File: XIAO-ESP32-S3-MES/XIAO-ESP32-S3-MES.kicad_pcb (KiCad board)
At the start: 2 copper layers, 36 x 39 mm, 11 parts, among them SW1 Conn_01x02_Socket, U2 XIAO-ESP32-S3-SMD

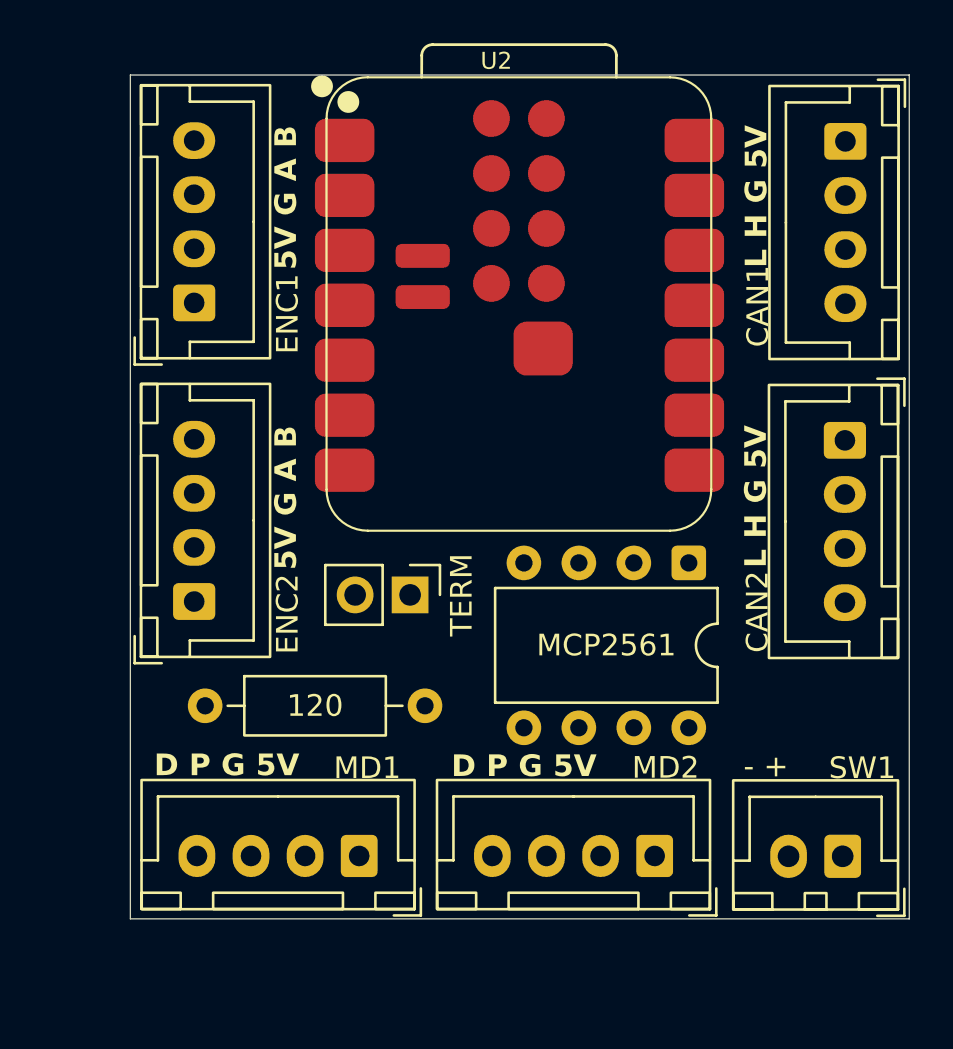
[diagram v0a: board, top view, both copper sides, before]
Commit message: MES配置完了
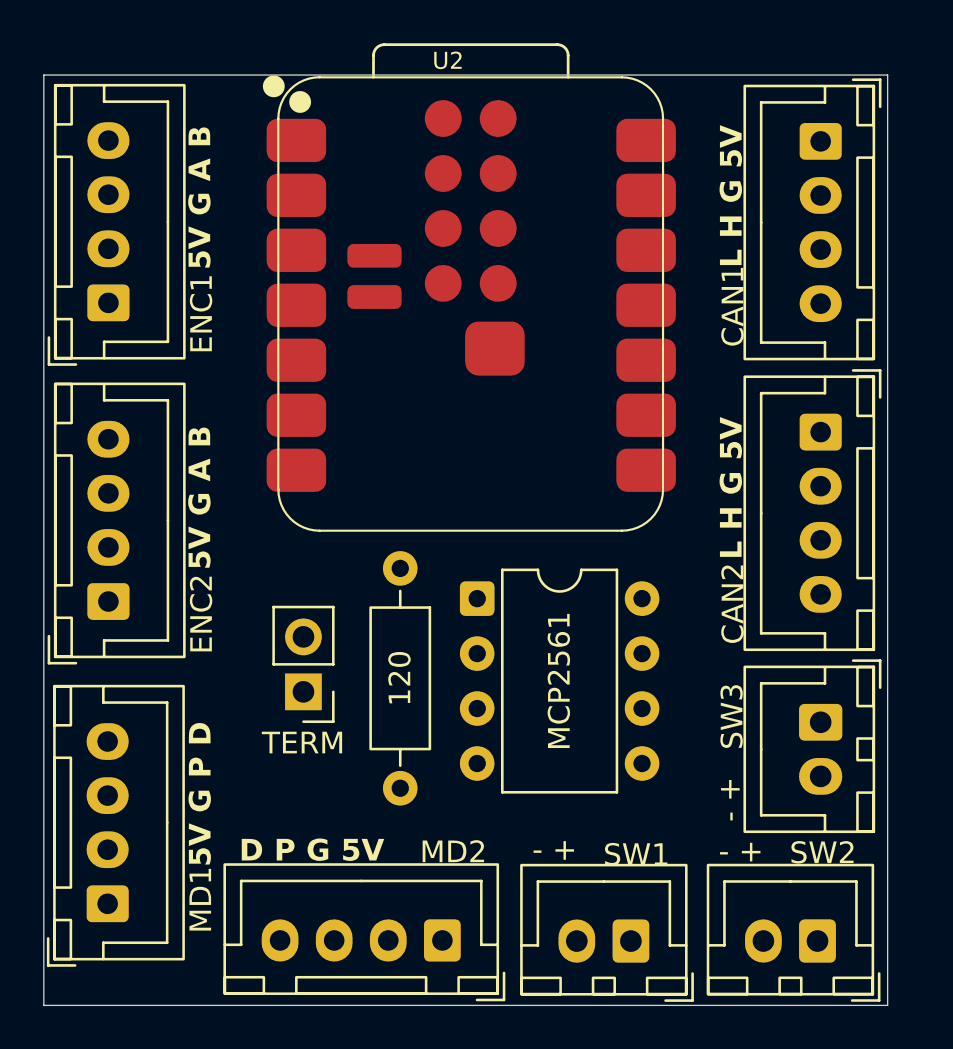
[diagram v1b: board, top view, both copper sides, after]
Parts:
- added SW2: SW2, Connector_JST:JST_XH_B2B-XH-A_1x02_P2.50mm_Vertical, F.Cu at (128.8, 92.0)
- added SW3: SW3, Connector_JST:JST_XH_B2B-XH-A_1x02_P2.50mm_Vertical, F.Cu at (128.9, 81.9)
- SW1: value Conn_01x02_Socket -> SW1
- moved MD1 11.8 mm to (96.0, 90.3), turned to 90 degrees
- moved R1 11.0 mm to (109.5, 74.8), turned to -90 degrees
- moved MD2 10.6 mm to (111.4, 92.0)
- moved SW1 10.5 mm to (120.1, 92.0)
- moved U1 9.92 mm to (113.0, 76.2), turned to 0 degrees
- moved TERM 6.66 mm to (105.0, 80.5), turned to 180 degrees
- moved ENC1 3.96 mm to (96.0, 62.5)
- moved ENC2 3.96 mm to (96.0, 76.3)
- moved U2 2.23 mm to (103.8, 73.1)
- moved CAN2 1.18 mm to (128.9, 68.5)
- moved CAN1 1.14 mm to (128.9, 55.1)
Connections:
- net ENC2_A renamed ENC2_A/SW2
- net ENC2_B renamed ENC2_B/SW3
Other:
- board size 36 x 39 mm -> 39 x 43 mm
- board text added: "5V G P D"
- board text added: "XIAO ESP32-S3 NHK2027 MES v1.0"
- board text removed: "XIAO ESP32-S3 MES v1.0"
